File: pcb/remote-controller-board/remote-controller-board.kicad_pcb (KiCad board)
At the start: 2 copper layers, 71.1 x 40.6 mm, 10 parts, among them J1 Conn_01x07, J2 Conn_01x05, SW1 SW_Push, SW2 SW_Push, SW3 SW_Push, SW4 SW_Push

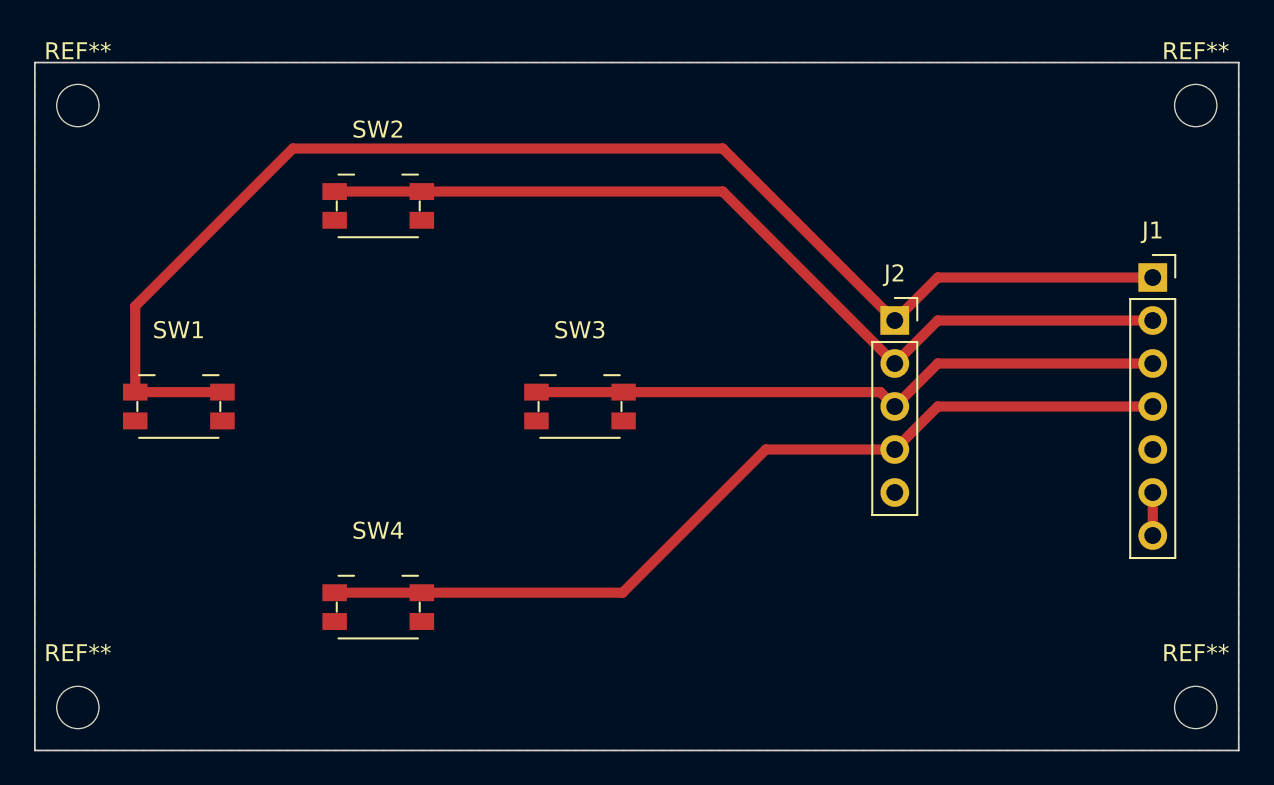
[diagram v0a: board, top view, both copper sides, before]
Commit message: New PCB & case
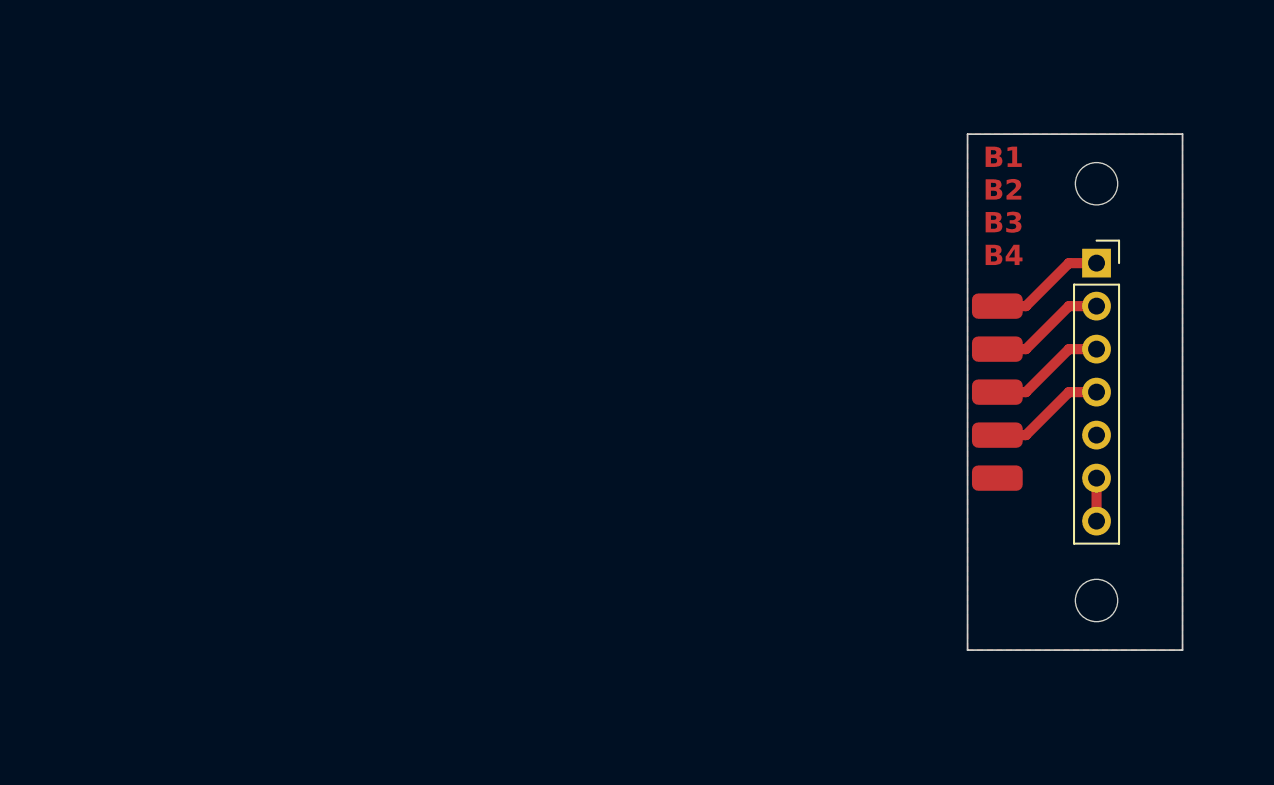
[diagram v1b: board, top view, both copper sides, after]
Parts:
- removed the REF** at (117.6, 115.2)
- removed the REF** at (183.7, 79.6)
- removed the REF** at (183.7, 115.2)
- removed the REF** at (117.6, 79.6)
- removed SW1, SW2, SW3, SW4: SW_Push, Button_Switch_SMD:Panasonic_EVQPUM_EVQPUD
- added REF**: MountingHole_2.5mm, MountingHole:MountingHole_2.5mm, F.Cu at (177.8, 84.2)
- added REF**: MountingHole_2.5mm, MountingHole:MountingHole_2.5mm, F.Cu at (177.8, 108.8)
- J2: footprint Connector_PinSocket_2.54mm:PinSocket_1x05_P2.54mm_Vertical -> Custom:Conn_01x05
- moved J2 7.39 mm to (171.9, 96.5), turned to -90 degrees
- moved J1 3.43 mm to (177.8, 88.9)
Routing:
- net RE1: track 79.5 -> 6.91 mm
- net RE2: track 53.6 -> 6.91 mm
- net RE4: track 52.9 -> 6.91 mm
- net RE3: track 37.8 -> 6.91 mm
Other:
- board size 71.1 x 40.6 mm -> 12.7 x 30.5 mm
- board text added: "B1 B2 B3 B4"
